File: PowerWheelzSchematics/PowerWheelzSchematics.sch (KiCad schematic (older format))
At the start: 14 parts

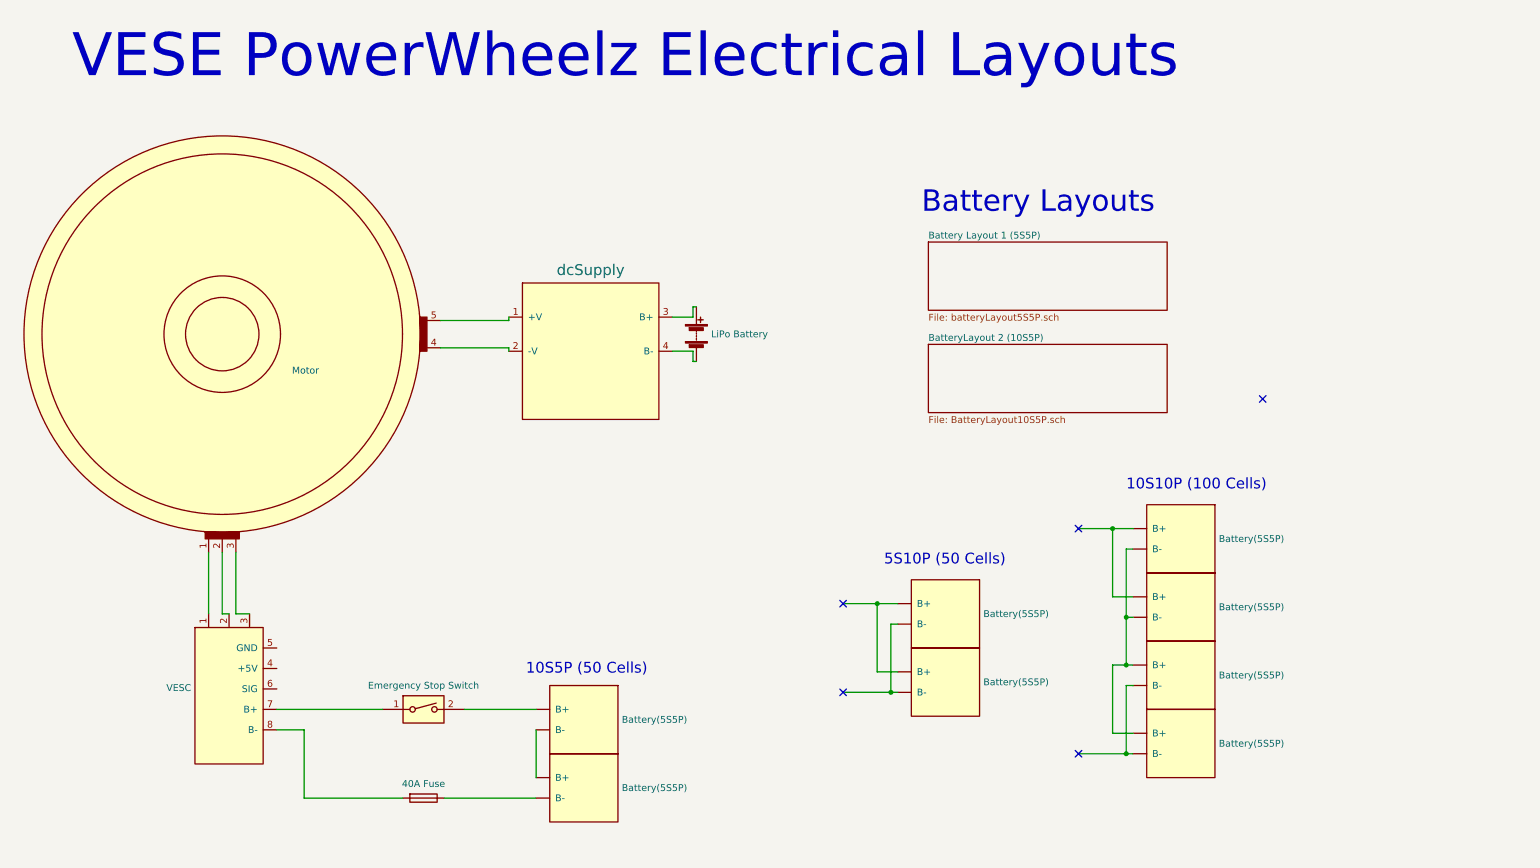
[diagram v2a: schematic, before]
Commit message: Update
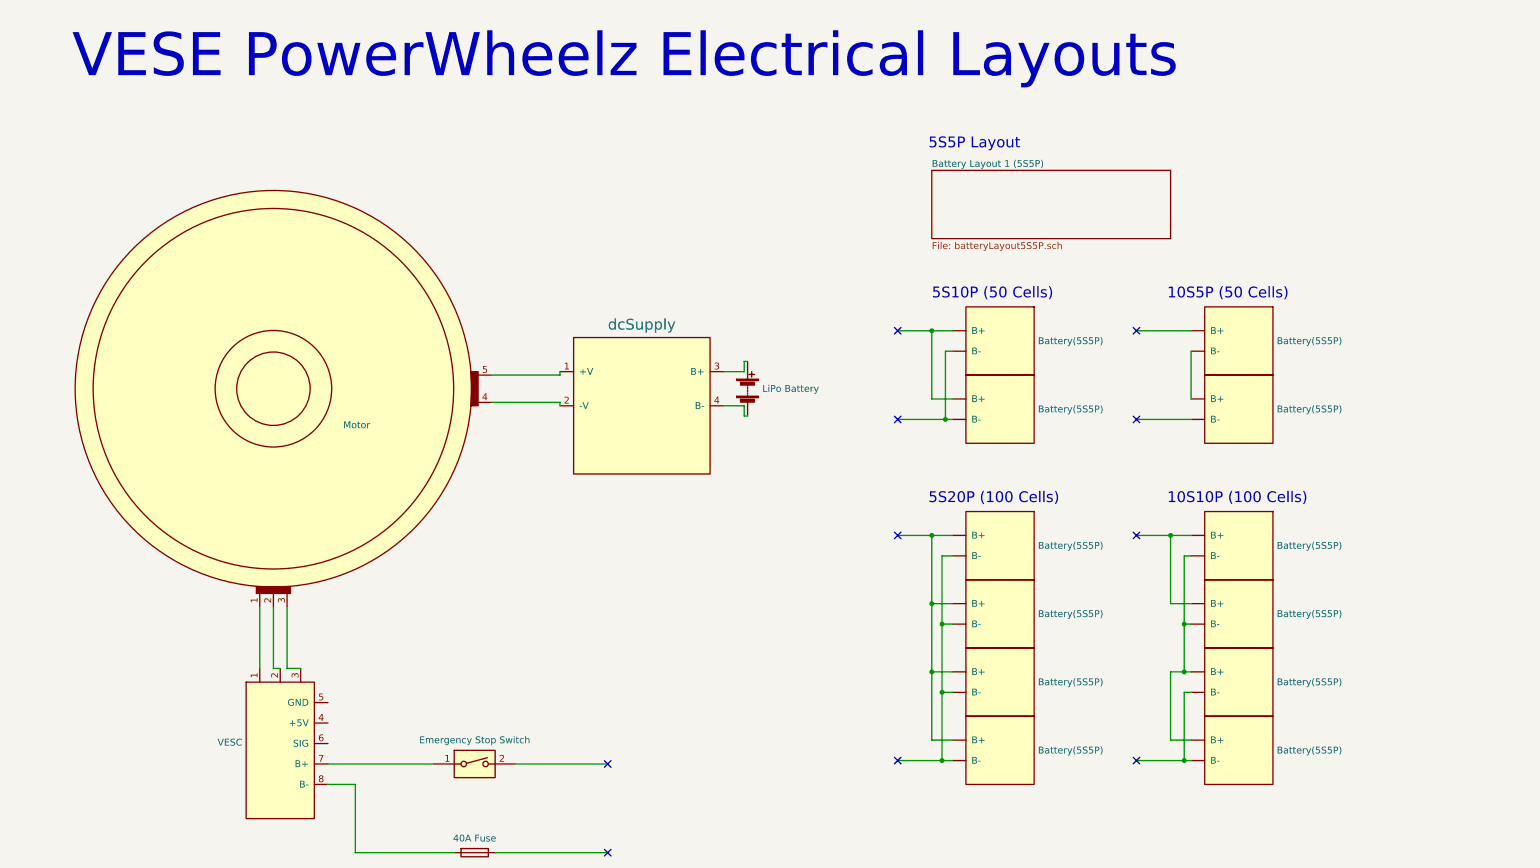
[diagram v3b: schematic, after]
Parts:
- added U? (x4): Battery(5S5P), symbol VESE:Battery(5S5P)
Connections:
- net at U?.~ (B-), U?.~ (B-): now also U?.~ (B-), U?.~ (B-)
- net at U?.~ (B-), U?.~ (B-): no longer U?.~ (B-), U?.~ (B-)
- net at SW?.2: no longer U?.~ (B-)
- net at F.1: no longer U?.~ (B-)
- new net: U?.~ (B-), U?.~ (B-), U?.~ (B-), U?.~ (B-) (x2)
- new net: U?.~ (B-), U?.~ (B-) (x2)
- no-connect marks 5 -> 10
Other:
- note added: "5S20P (100 Cells)"
- note added: "5S5P Layout"
- note removed: "Battery Layouts"
